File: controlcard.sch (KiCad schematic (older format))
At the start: 1 part

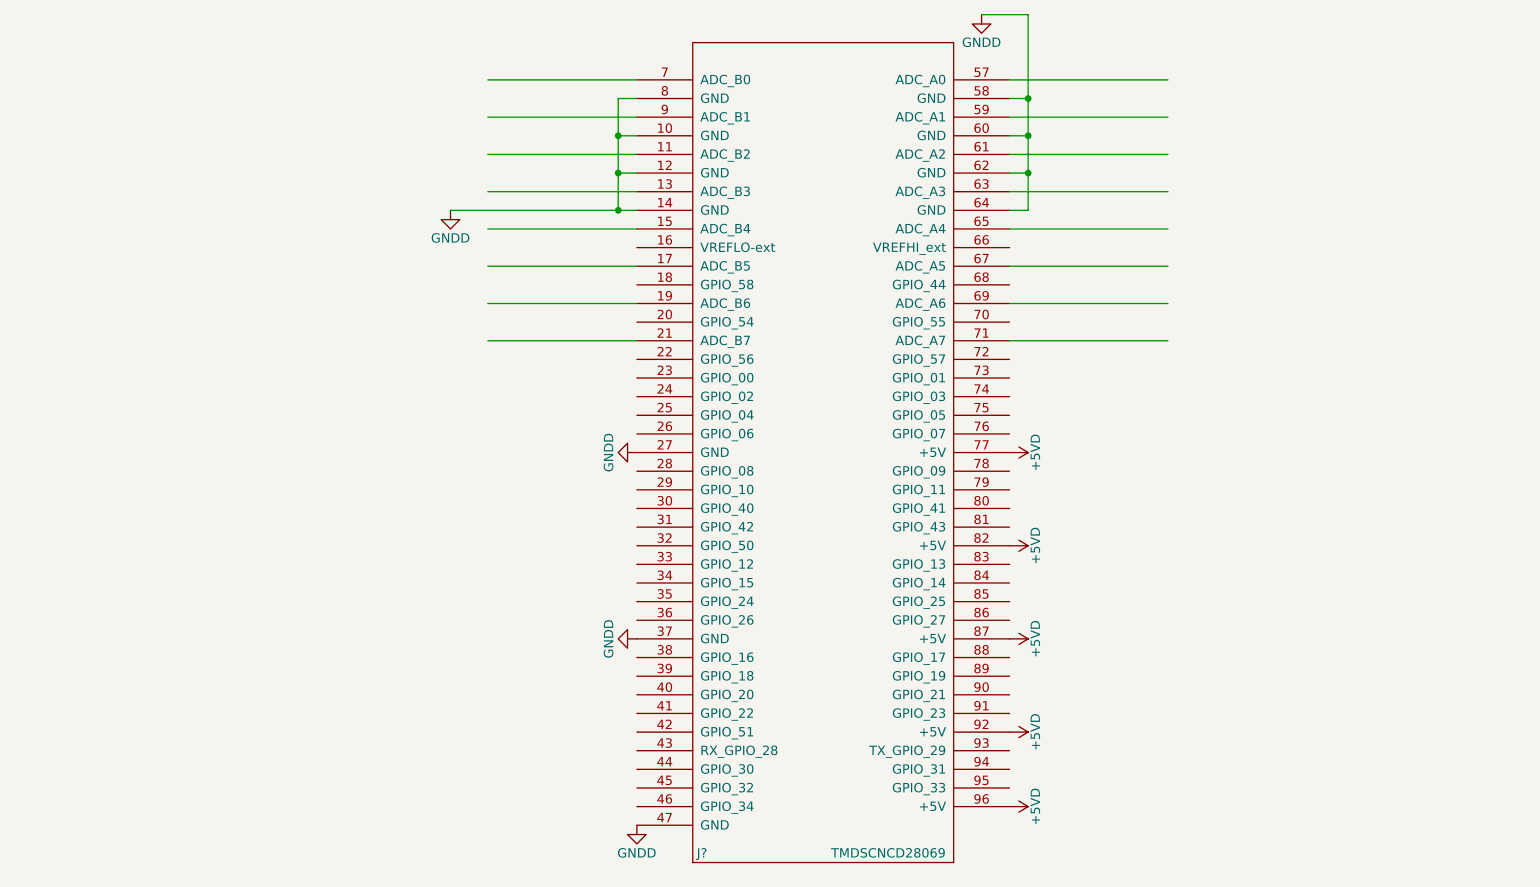
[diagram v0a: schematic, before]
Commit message: V0 schematic complete (?)
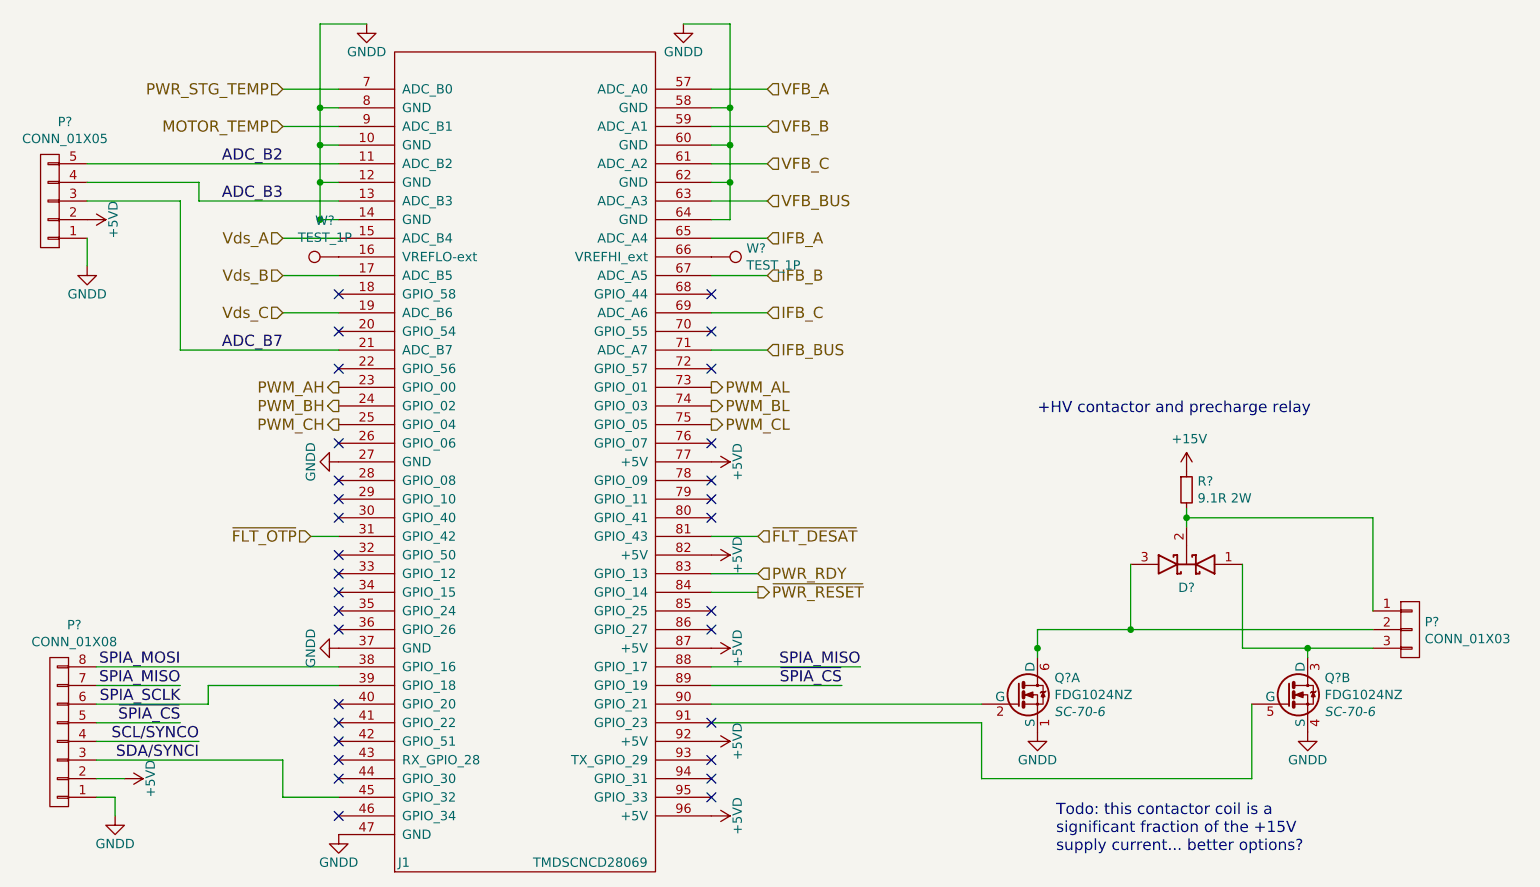
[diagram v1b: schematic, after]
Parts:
- added D?: D_Schottky_x2_KCom_AKA, symbol D_Schottky_x2_KCom_AKA
- added P?: CONN_01X03, symbol CONN_01X03
- added P?: CONN_01X05, symbol CONN_01X05
- added P?: CONN_01X08, symbol CONN_01X08
- added Q? (x2): FDG1024NZ, SC-70-6, symbol FDG1024NZ
- added R?: 9.1R 2W, symbol R_Small
- added W? (x2): TEST_1P, symbol TEST_1P
- gave numbers to parts that had none: 1
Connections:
- net labels added: +15V, ADC_B2, ADC_B3, ADC_B7, IFB_A, IFB_B, IFB_BUS, IFB_C, MOTOR_TEMP, PWM_AH, PWM_AL, PWM_BH, PWM_BL, PWM_CH, PWM_CL, PWR_RDY, PWR_STG_TEMP, SCL/SYNCO, SDA/SYNCI, SPIA_MISO, SPIA_MOSI, SPIA_SCLK, VFB_A, VFB_B, VFB_BUS, VFB_C, Vds_A, Vds_B, Vds_C, ~FLT_DESAT, ~FLT_OTP, ~PWR_RESET, ~SPIA_CS
- wire segments 27 -> 66
- no-connect marks 0 -> 31
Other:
- note added: "+HV contactor and precharge relay"
- note added: "Todo: this contactor coil is a\nsignificant fraction of the +15V\nsupply current... better options?"
- moved on the sheet: J1
